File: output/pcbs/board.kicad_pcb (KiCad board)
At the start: 2 copper layers, 95 x 86 mm, 38 parts

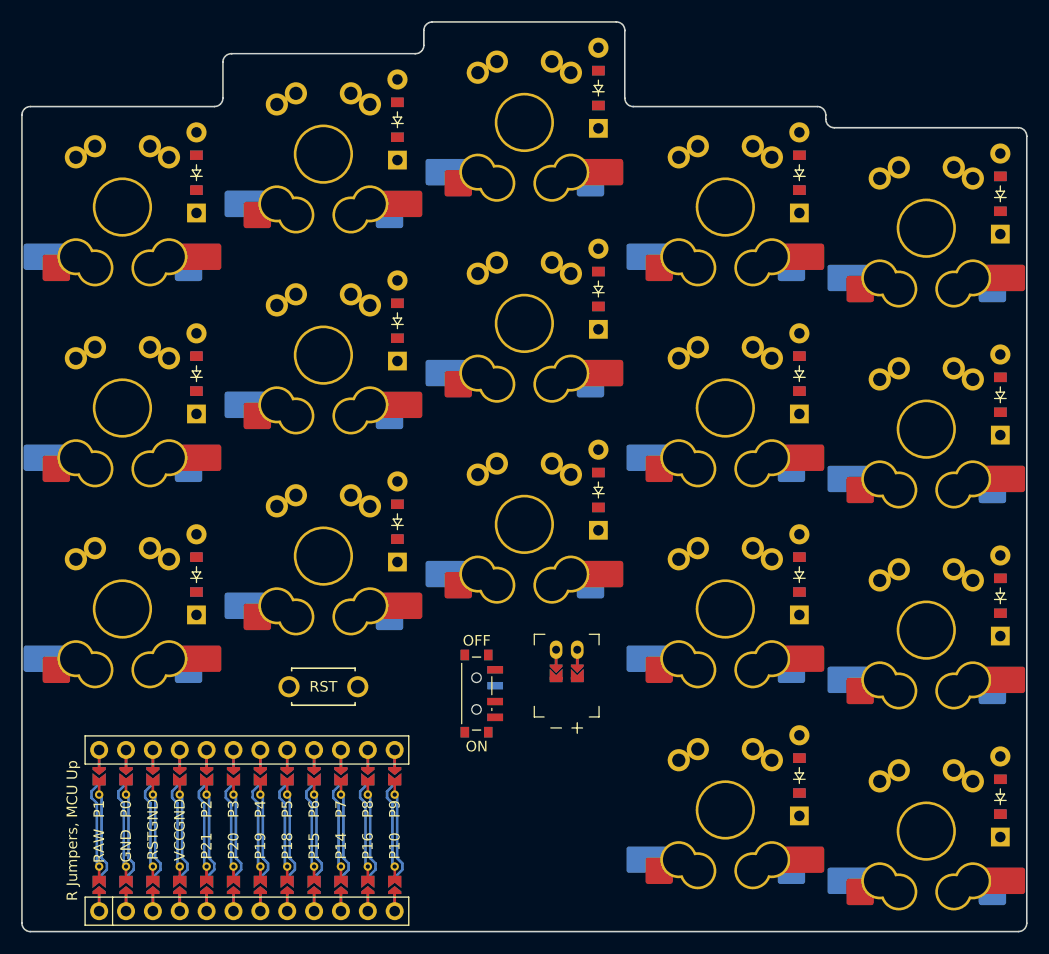
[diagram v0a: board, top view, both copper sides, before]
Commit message: mk12 config
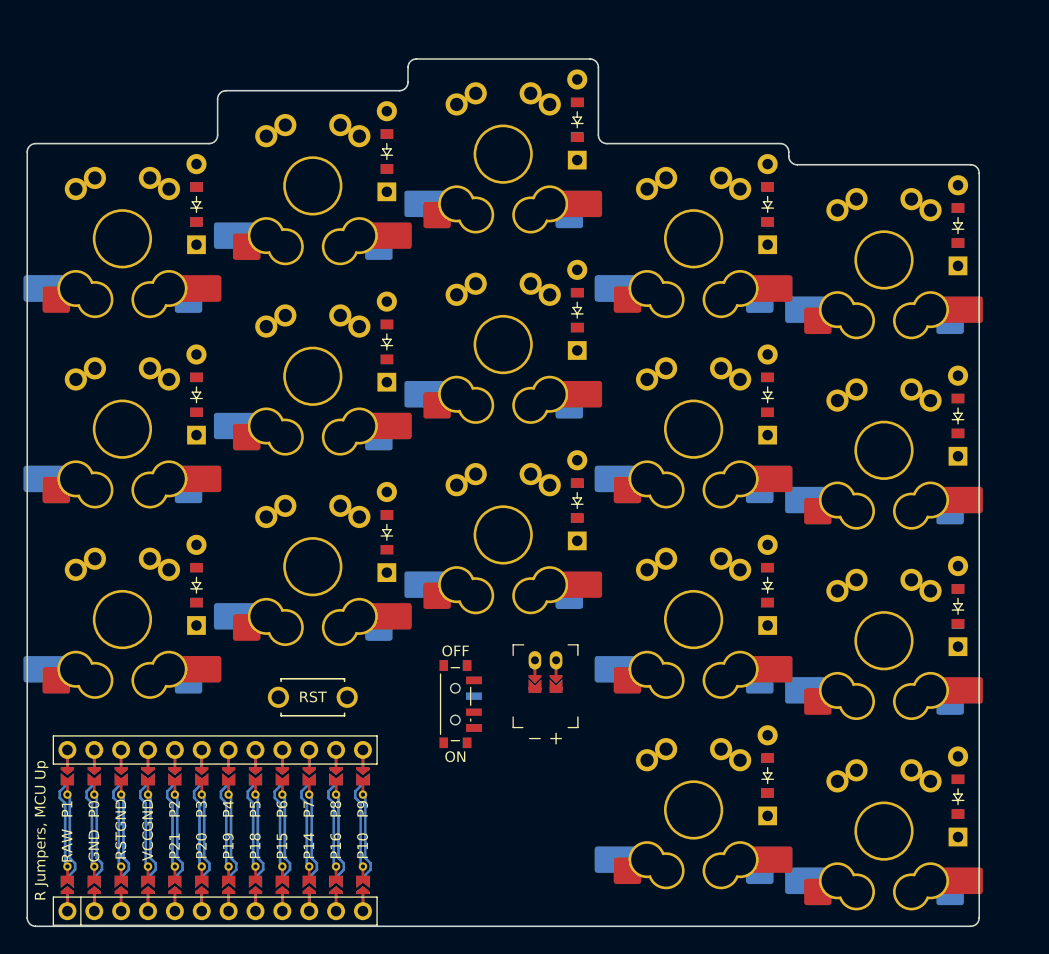
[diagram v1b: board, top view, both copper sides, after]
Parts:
- moved D17 5.00 mm to (254.0, 119.8)
- moved S17 5.00 mm to (247.0, 123.0)
- moved D16 4.47 mm to (254.0, 137.8)
- moved S16 4.47 mm to (247.0, 141.0)
- moved D13 4.24 mm to (236.0, 117.8)
- moved S13 4.24 mm to (229.0, 121.0)
- moved D15 4.12 mm to (254.0, 155.8)
- moved S15 4.12 mm to (247.0, 159.0)
- moved D14 4.00 mm to (254.0, 173.8)
- moved S14 4.00 mm to (247.0, 177.0)
- moved D12 3.61 mm to (236.0, 135.8)
- moved D9 3.61 mm to (218.0, 109.8)
- moved S12 3.61 mm to (229.0, 139.0)
- moved S9 3.61 mm to (211.0, 113.0)
- moved D11 3.16 mm to (236.0, 153.8)
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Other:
- board size 95 x 86 mm -> 90 x 82 mm

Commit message: mk3 pcb donw
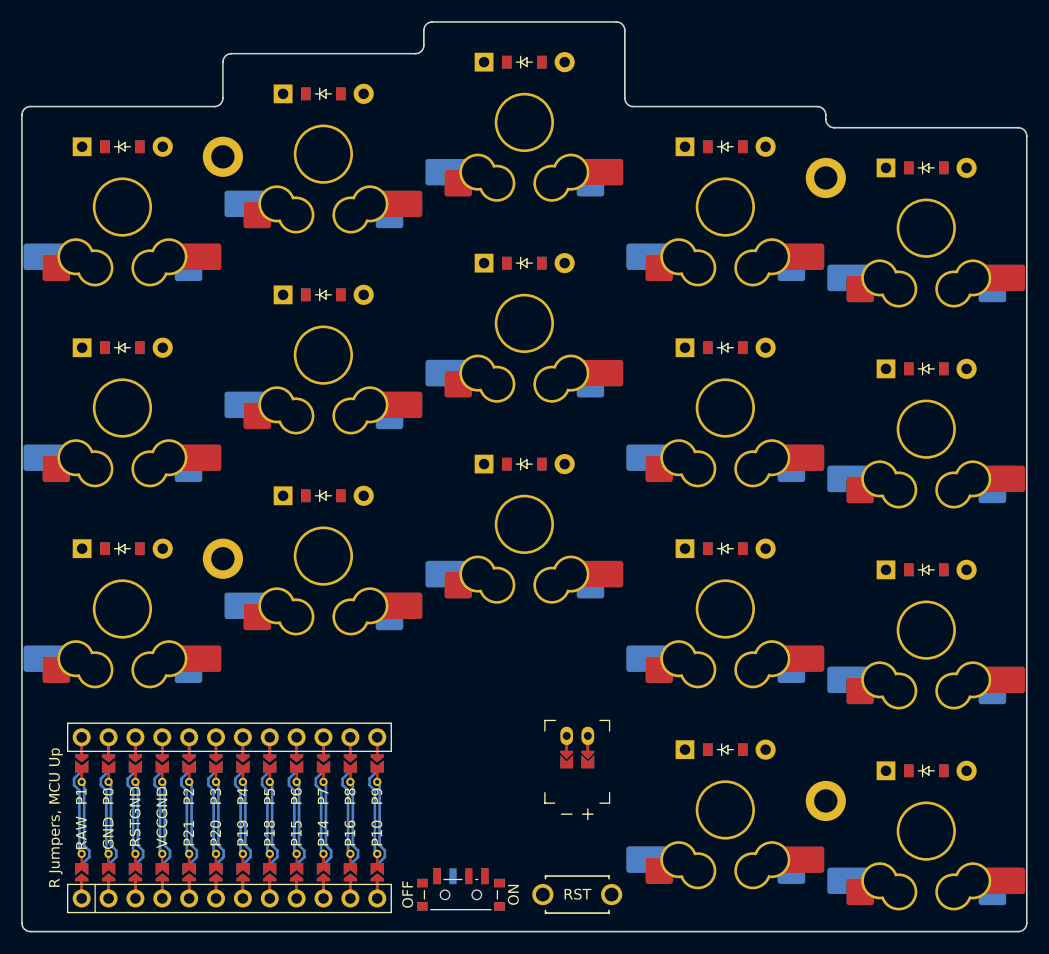
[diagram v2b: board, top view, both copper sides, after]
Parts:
- added H1: , ceoloide:mounting_hole_plated, F.Cu at (184.5, 113.2)
- added H2: , ceoloide:mounting_hole_plated, F.Cu at (184.5, 151.2)
- added H3: , ceoloide:mounting_hole_plated, F.Cu at (241.5, 115.2)
- added H4: , ceoloide:mounting_hole_plated, F.Cu at (241.5, 174.2)
- moved RST1 31.2 mm to (218.0, 183.0)
- moved PWR1 18.0 mm to (207.0, 183.0), turned to -90 degrees
- moved D3 8.87 mm to (175.0, 112.3), turned to 0 degrees
- moved D2 8.29 mm to (175.0, 131.3), turned to 0 degrees
- moved D6 8.11 mm to (194.0, 107.3), turned to 0 degrees
- moved D1 7.80 mm to (175.0, 150.3), turned to 0 degrees
- moved JST1 7.75 mm to (218.0, 168.0)
- moved D5 7.47 mm to (194.0, 126.3), turned to 0 degrees
- moved D9 7.40 mm to (213.0, 104.3), turned to 0 degrees
- moved D4 6.92 mm to (194.0, 145.3), turned to 0 degrees
- moved D13 6.76 mm to (232.0, 112.3), turned to 0 degrees
- moved D8 6.69 mm to (213.0, 123.3), turned to 0 degrees
- moved D17 6.22 mm to (251.0, 114.3), turned to 0 degrees
- moved D7 6.07 mm to (213.0, 142.3), turned to 0 degrees
- moved D12 5.98 mm to (232.0, 131.3), turned to 0 degrees
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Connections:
- D1 pad 1: P14 -> P16
- D10 pad 1: P15 -> P10
- D11 pad 1: P14 -> P16
- D12 pad 1: P16 -> P14
- D13 pad 1: P10 -> P15
- D14 pad 1: P15 -> P10
- D15 pad 1: P14 -> P16
- D16 pad 1: P16 -> P14
- D17 pad 1: P10 -> P15
- D2 pad 1: P16 -> P14
- D3 pad 1: P10 -> P15
- D4 pad 1: P14 -> P16
- D5 pad 1: P16 -> P14
- D6 pad 1: P10 -> P15
- D7 pad 1: P14 -> P16
- D8 pad 1: P16 -> P14
- D9 pad 1: P10 -> P15
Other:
- board size 90 x 82 mm -> 95 x 86 mm
